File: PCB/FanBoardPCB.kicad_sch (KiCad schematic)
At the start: 29 parts, among them J1 FAN3, J13 FanBrdConn, J2 FAN4, J3 FAN1, J4 FAN2, Q1 IRLML0030, Q2 IRLML0030, Q3 IRLML0030, Q4 IRLML0030

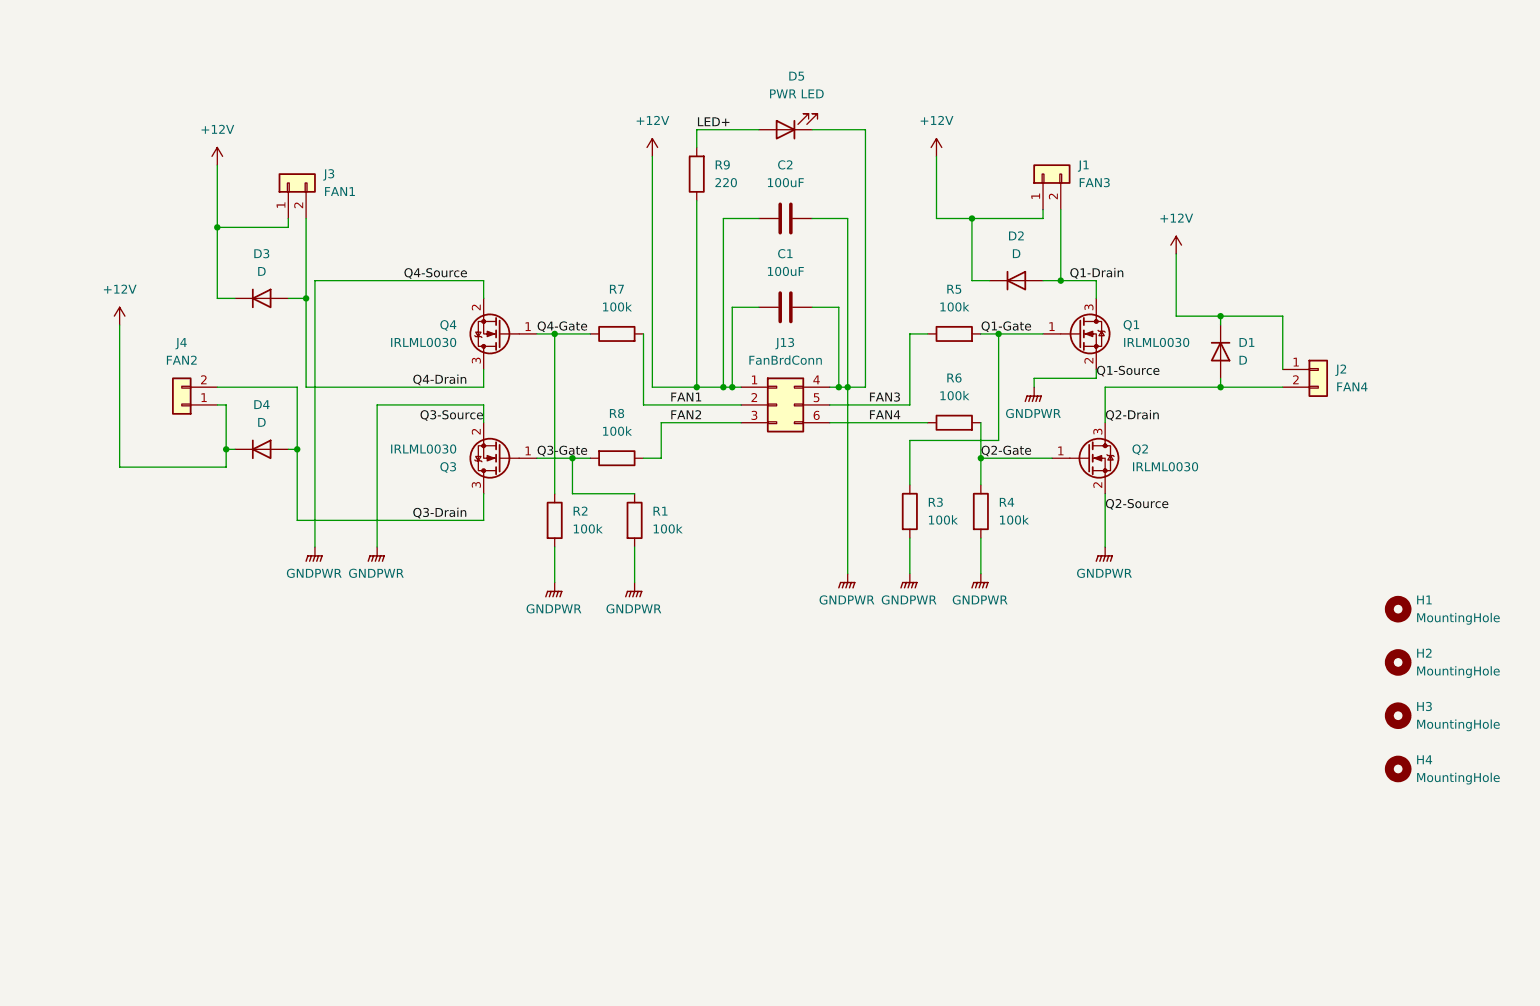
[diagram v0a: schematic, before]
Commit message: cleanup PCB
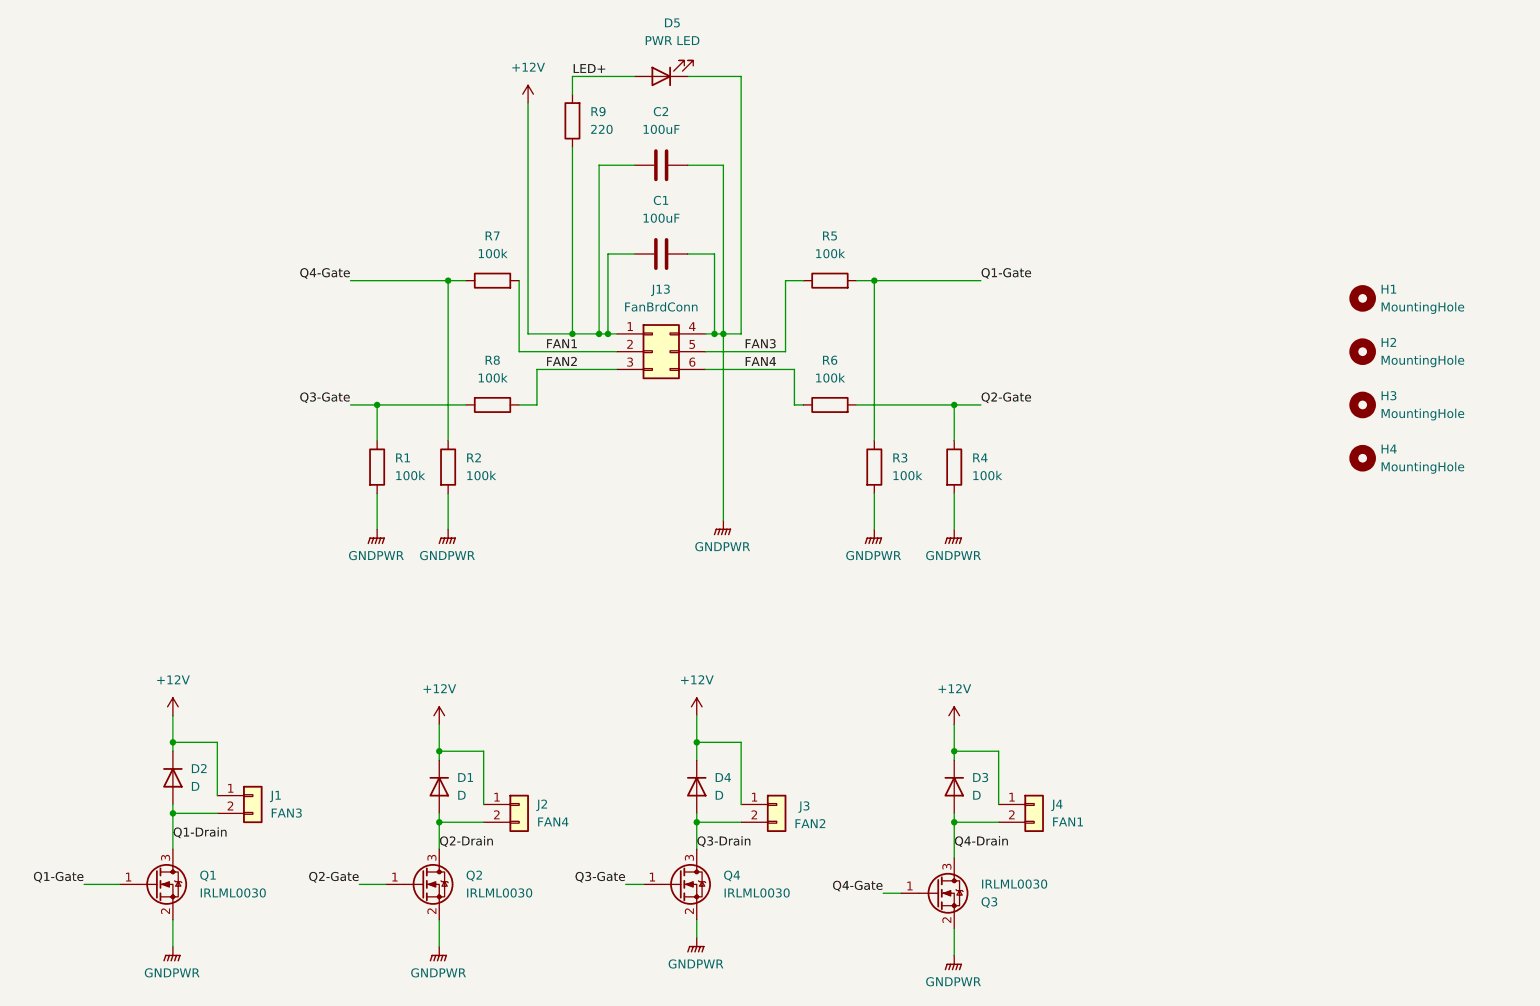
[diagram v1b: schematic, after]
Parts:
- J3: value FAN1 -> FAN2
- J4: value FAN2 -> FAN1
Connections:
- net Q3-Drain: now also J3.2 (Pin_2), Q4.3 (D); no longer J4.2 (Pin_2), Q3.3 (D)
- net Q3-Gate: now also Q4.1 (G); no longer Q3.1 (G)
- net Q4-Drain: now also J4.2 (Pin_2), Q3.3 (D); no longer J3.2 (Pin_2), Q4.3 (D)
- net Q4-Gate: now also Q3.1 (G); no longer Q4.1 (G)
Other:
- moved on the sheet: C1, C2, D1, D5, H1, H2, H3, H4, J1, J13, J2, Q1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
